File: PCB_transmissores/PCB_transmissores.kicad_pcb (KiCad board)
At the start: 2 copper layers, 120.1 x 80 mm, 17 parts, among them J2 Barrel_Jack_MountingPin

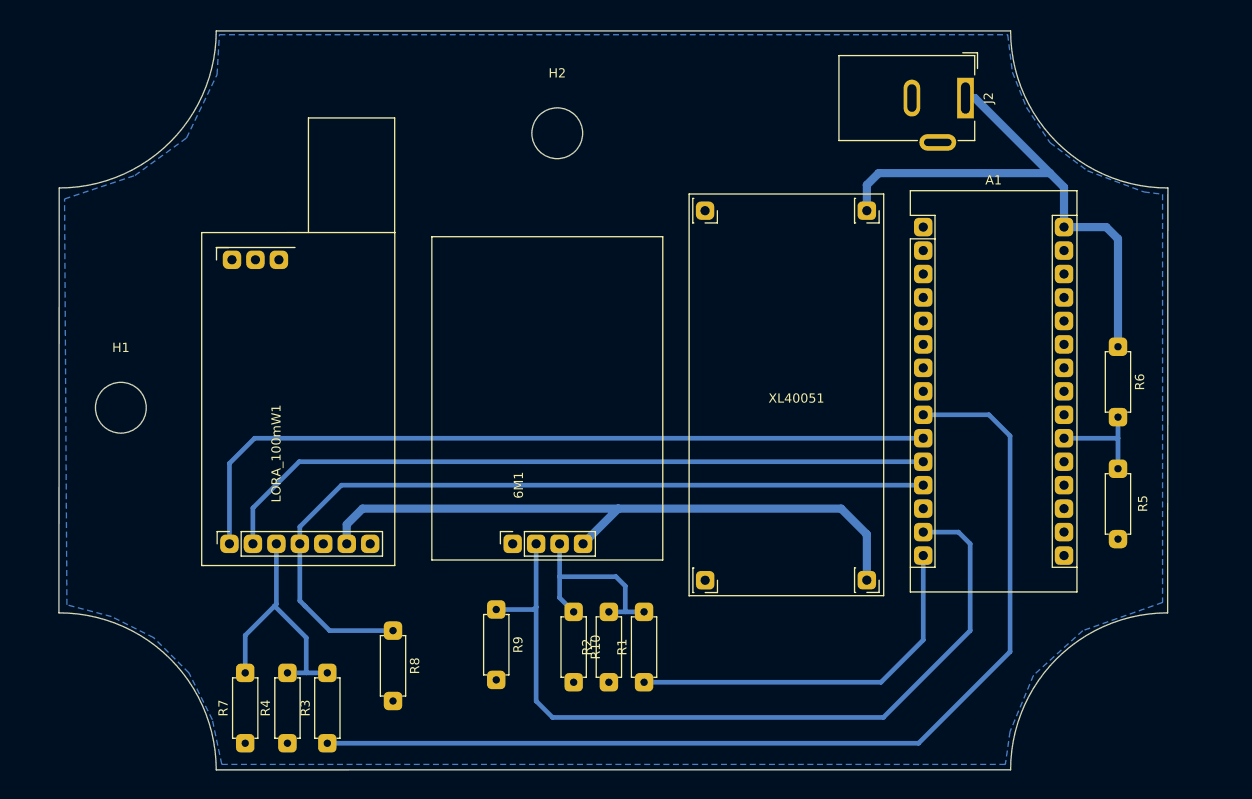
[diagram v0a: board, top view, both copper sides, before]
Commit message: Atualização placa dos transmissores
Up
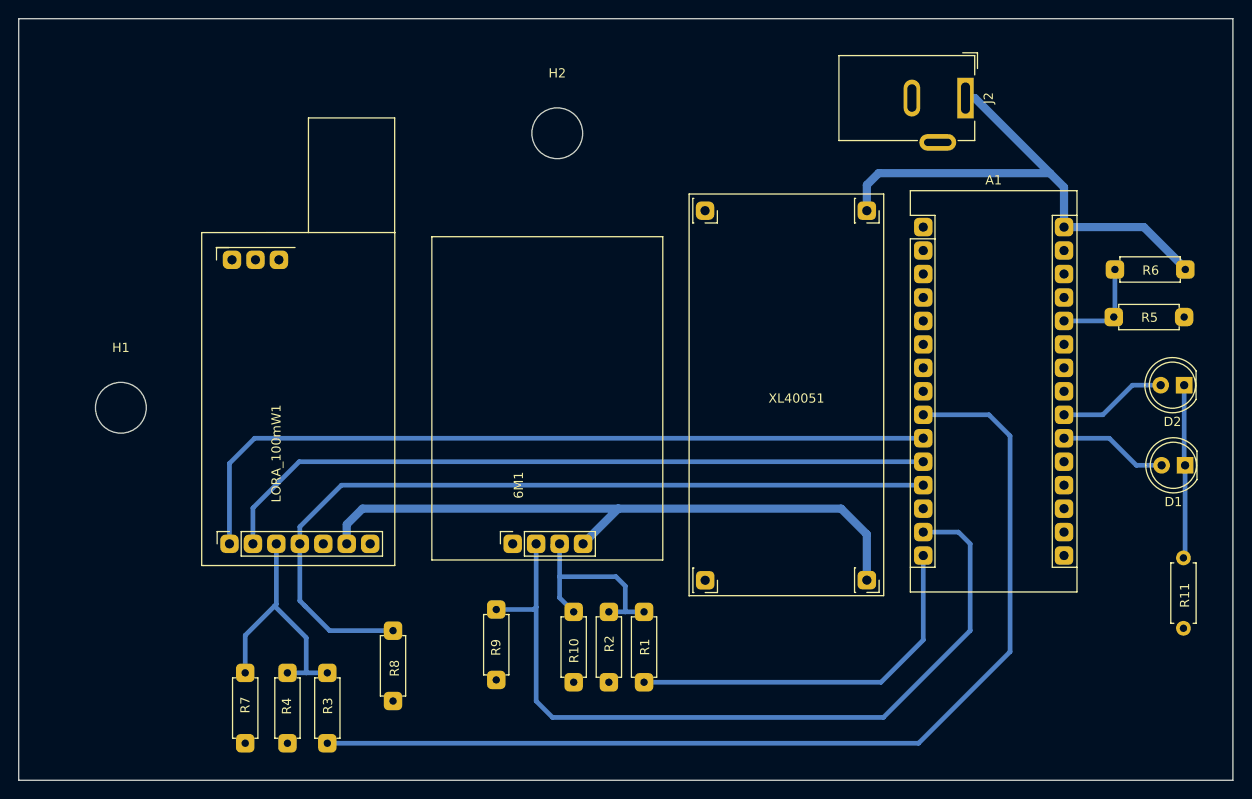
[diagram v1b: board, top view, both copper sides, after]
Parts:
- added D1: LED, LED_THT:LED_D5.0mm, F.Cu at (206.4, 110.6)
- added D2: LED, LED_THT:LED_D5.0mm, F.Cu at (206.3, 102.0)
- added R11: 100, Resistor_THT:R_Axial_DIN0207_L6.3mm_D2.5mm_P7.62mm_Horizontal, F.Cu at (206.2, 120.7)
- R1, R3: value 1k -> 240
- R2, R4: value 0,5k -> 560
- R6: value 36k -> 10k
- moved R5 25.1 mm to (206.3, 94.6), turned to 180 degrees
- moved R6 11.1 mm to (206.4, 89.4), turned to 180 degrees
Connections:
- A1 pad 22: Net-(A1-Pad22) -> A3
- A1 pad 26: Net-(A1-Pad26) -> A7
- R5 pad 2: A2 -> A7
- R6 pad 2: A2 -> A7
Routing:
- net R11: track 0.00 -> 18.8 mm
- net A3: track 0.00 -> 11.8 mm
- net A7: track 0.00 -> 10.8 mm
- net VIN: track 60.2 -> 57.2 mm
- removed copper zone on B.Cu, net GND
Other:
- board size 120.1 x 80 mm -> 131.4 x 82.4 mm
